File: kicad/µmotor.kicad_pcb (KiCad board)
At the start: 2 copper layers, 20 x 20 mm, 31 parts, among them J101 CAN+PWR, J201 TX, J202 RX, J203 SWDIO, J204 SWCLK, J205 GND, J501 1, J502 2, U201 STM32F042F6Px, U301 MCP1700T-3002E/TT, U401 AS5045B, U501 DRV8870, U502 INA180A1, U601 TCAN330

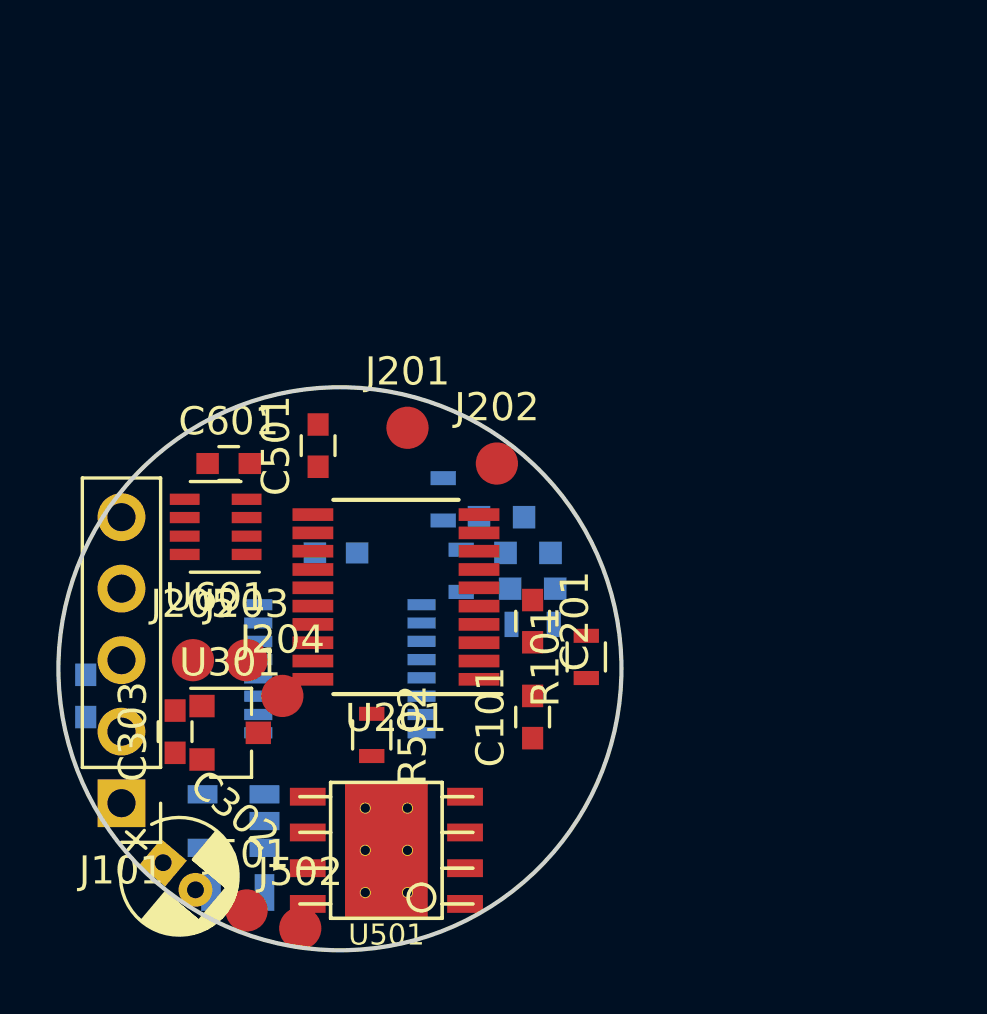
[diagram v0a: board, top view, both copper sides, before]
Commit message: layout: components placed
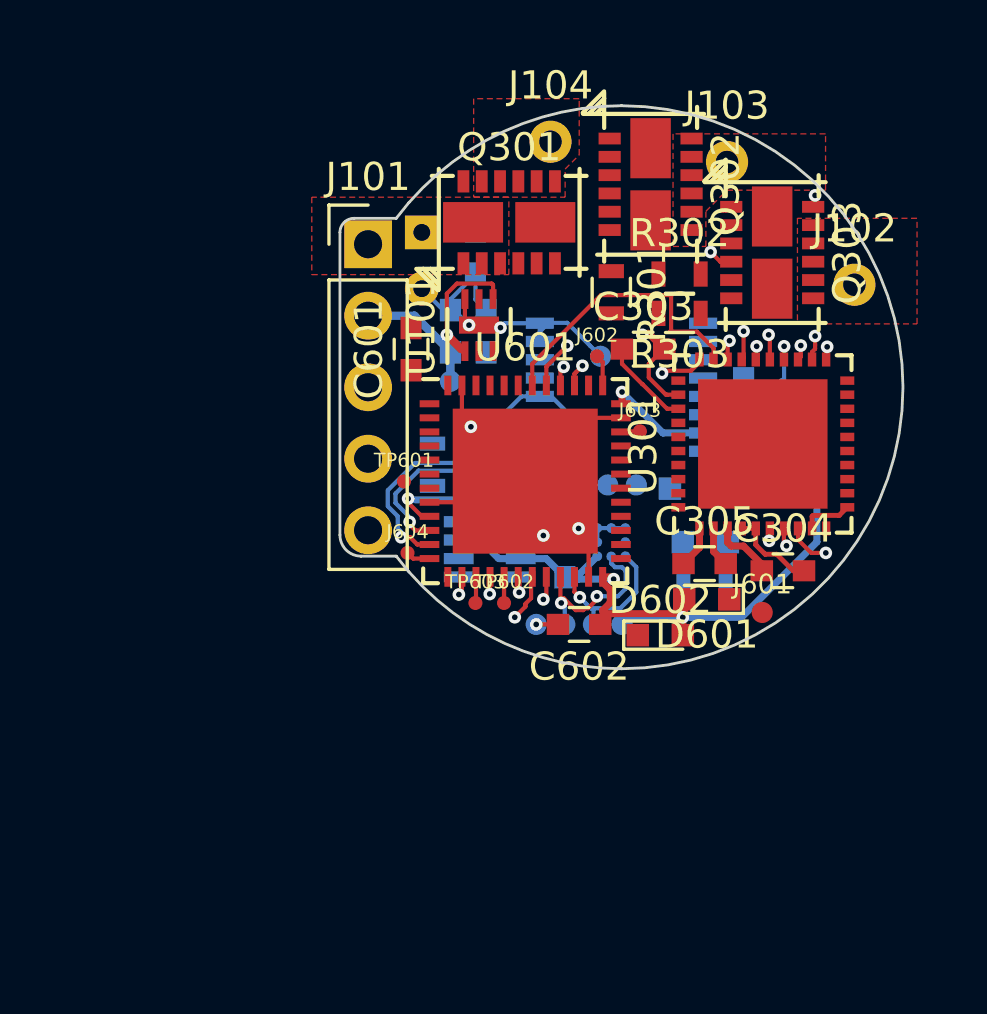
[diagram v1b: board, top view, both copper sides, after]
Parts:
- removed C501: NC, Capacitors_SMD:C_0603
- removed D401: Red, LEDs:LED_0603
- removed D402: Yellow, LEDs:LED_0603
- removed J205: GND, Measurement_Points:Measurement_Point_Round-SMD-Pad_Small
- removed R101: 100k, Resistors_SMD:R_0603
- removed R401, R402: 1k, Resistors_SMD:R_0603
- removed R501: 150m, Resistors_SMD:R_0805
- removed R502: 0, Resistors_SMD:R_0603
- removed U502: INA180A1, TO_SOT_Packages_SMD:SOT-23-5
- added C102: 1µ 6V3, Capacitors_SMD:C_0603, B.Cu at (155.2, 88.0)
- added C304: 1µ 16V X7R, Capacitors_SMD:C_0603, F.Cu at (165.7, 96.5)
- added C305: 47n 50V X7R, Capacitors_SMD:C_0603, F.Cu at (163.0, 96.3)
- added C602: 100n, Capacitors_SMD:C_0603, F.Cu at (158.5, 98.4)
- added D202: Yellow, LEDs:LED_0603, B.Cu at (162.5, 93.6)
- added D601: Blue, LEDs:LED_0603, F.Cu at (163.0, 97.5)
- added D602: Red, LEDs:LED_0603, F.Cu at (161.4, 98.8)
- added J102: U, Measurement_Points:Measurement_Point_Round-TH_Small, F.Cu at (168.3, 86.4)
- added J103: V, Measurement_Points:Measurement_Point_Round-TH_Small, F.Cu at (163.8, 82.0)
- added J104: W, Measurement_Points:Measurement_Point_Round-TH_Small, F.Cu at (157.5, 81.3)
- added J105: U, Measurement_Point_Round-SMD-Pad_Smaller:Measurement_Point_Round-SMD-Pad_Smaller_0.75mm, B.Cu at (160.5, 93.5)
- added J106: V, Measurement_Point_Round-SMD-Pad_Smaller:Measurement_Point_Round-SMD-Pad_Smaller_0.75mm, B.Cu at (159.5, 93.5)
- added J107: W, Measurement_Point_Round-SMD-Pad_Smaller:Measurement_Point_Round-SMD-Pad_Smaller_0.75mm, B.Cu at (158.5, 93.5)
- added J503: 3V3, Measurement_Point_Round-SMD-Pad_Smaller:Measurement_Point_Round-SMD-Pad_Smaller_0.75mm, B.Cu at (160.0, 98.4)
- added J504: GND, Measurement_Point_Round-SMD-Pad_Smaller:Measurement_Point_Round-SMD-Pad_Smaller_0.75mm, B.Cu at (157.0, 98.4)
- added J601: GND, Measurement_Point_Round-SMD-Pad_Smaller:Measurement_Point_Round-SMD-Pad_Smaller_0.75mm, F.Cu at (165.0, 98.0)
- added J602: SWCLK, Measurement_Point_Round-SMD-Pad_Smaller:Measurement_Point_Round-SMD-Pad_Smaller_0.5mm, F.Cu at (159.1, 88.9)
- added J603: SWDIO, Measurement_Point_Round-SMD-Pad_Smaller:Measurement_Point_Round-SMD-Pad_Smaller_0.5mm, F.Cu at (160.7, 91.6)
- added J604: TX, Measurement_Point_Round-SMD-Pad_Smaller:Measurement_Point_Round-SMD-Pad_Smaller_0.5mm, F.Cu at (152.4, 95.9)
- added Q301: FDMD82xx, DFN-12-2EP_3.3x5mm_Pitch0.65mm:DFN-12-2EP_3.3x5mm_Pitch0.65mm, F.Cu at (156.0, 84.1)
- added Q302: FDMD82xx, DFN-12-2EP_3.3x5mm_Pitch0.65mm:DFN-12-2EP_3.3x5mm_Pitch0.65mm, F.Cu at (161.0, 82.8)
- added Q303: FDMD82xx, DFN-12-2EP_3.3x5mm_Pitch0.65mm:DFN-12-2EP_3.3x5mm_Pitch0.65mm, F.Cu at (165.4, 85.2)
- added R202: 1k, Resistors_SMD:R_0603, B.Cu at (164.7, 93.1)
- added R301: 5m, Resistors_SMD:R_0603, F.Cu at (159.6, 86.6)
- added R302: 5m, Resistors_SMD:R_0603, F.Cu at (162.1, 86.0)
- added R303: 5m, Resistors_SMD:R_0603, F.Cu at (162.1, 87.4)
- added R601: 1k, Resistors_SMD:R_0603, B.Cu at (163.0, 96.9)
- added R602: 1k, Resistors_SMD:R_0603, B.Cu at (153.3, 92.8)
- added TP601: ~RST, Measurement_Point_Round-SMD-Pad_Smaller:Measurement_Point_Round-SMD-Pad_Smaller_0.5mm, F.Cu at (152.3, 93.3)
- added TP602: BK, Measurement_Point_Round-SMD-Pad_Smaller:Measurement_Point_Round-SMD-Pad_Smaller_0.5mm, F.Cu at (155.8, 97.7)
- added TP603: DAC, Measurement_Point_Round-SMD-Pad_Smaller:Measurement_Point_Round-SMD-Pad_Smaller_0.5mm, F.Cu at (154.8, 97.7)
- added U101: NCP4623HMX033TCG, Housings_DFN_QFN:DFN-6-1EP_2x2mm_Pitch0.5mm, F.Cu at (154.9, 87.8)
- C101: value 1u -> 1µ 16V; moved to B.Cu
- C201: moved to B.Cu
- C301: value 10µ/10V -> >10µ 35V; footprint Capacitors_SMD:C_0603 -> Capacitors_THT:CP_Radial_D4.0mm_P2.00mm
- C302: value 47µ/35V -> 100n 50V; footprint Capacitors_THT:CP_Radial_D4.0mm_P1.50mm -> Capacitors_SMD:C_0603; moved to B.Cu
- C303: value 10µ/6V3 -> 1µ 6V3 X7R
- D201: value Blue -> Red
- J201: value TX -> A; footprint Measurement_Points:Measurement_Point_Round-SMD-Pad_Small -> Measurement_Point_Round-SMD-Pad_Smaller:Measurement_Point_Round-SMD-Pad_Smaller_0.75mm; moved to B.Cu
- J202: value RX -> B; footprint Measurement_Points:Measurement_Point_Round-SMD-Pad_Small -> Measurement_Point_Round-SMD-Pad_Smaller:Measurement_Point_Round-SMD-Pad_Smaller_0.75mm; moved to B.Cu
- J203: value SWDIO -> 6V; footprint Measurement_Points:Measurement_Point_Round-SMD-Pad_Small -> Measurement_Point_Round-SMD-Pad_Smaller:Measurement_Point_Round-SMD-Pad_Smaller_0.75mm; moved to B.Cu
- J204: value SWCLK -> GND; footprint Measurement_Points:Measurement_Point_Round-SMD-Pad_Small -> Measurement_Point_Round-SMD-Pad_Smaller:Measurement_Point_Round-SMD-Pad_Smaller_0.75mm; moved to B.Cu
- J501: value 1 -> SCL; footprint Measurement_Points:Measurement_Point_Round-SMD-Pad_Small -> Measurement_Point_Round-SMD-Pad_Smaller:Measurement_Point_Round-SMD-Pad_Smaller_0.75mm; moved to B.Cu
- J502: value 2 -> SDA; footprint Measurement_Points:Measurement_Point_Round-SMD-Pad_Small -> Measurement_Point_Round-SMD-Pad_Smaller:Measurement_Point_Round-SMD-Pad_Smaller_0.75mm; moved to B.Cu
- U201: value STM32F042F6Px -> AS5045B; footprint Housings_SSOP:TSSOP-20_4.4x6.5mm_Pitch0.65mm -> Housings_SSOP:SSOP-16_4.4x5.2mm_Pitch0.65mm; moved to B.Cu
- U301: value MCP1700T-3002E/TT -> DRV8323S; footprint TO_SOT_Packages_SMD:SOT-23 -> Housings_DFN_QFN:QFN-40-1EP_6x6mm_Pitch0.5mm
- U401: value AS5045B -> TCAN330; footprint Housings_SSOP:SSOP-16_4.4x5.2mm_Pitch0.65mm -> TO_SOT_Packages_SMD:SOT-23-8
- U501: value DRV8870 -> TMP006; footprint HSOP-8:HSOP-8 -> WCSP-8_1.6x1.6mm_P0.5mm:WCSP-8_1.6x1.6mm_P0.5mm; moved to B.Cu
- U601: value TCAN330 -> STM32L433C(B-C)Ux_u; footprint TO_SOT_Packages_SMD:SOT-23-8 -> Housings_DFN_QFN:QFN-48-1EP_7x7mm_Pitch0.5mm
- moved C302 24.3 mm to (154.8, 85.2), turned to 270 degrees
- moved J101 21.7 mm to (151.0, 84.9), turned to 0 degrees
- moved U301 21.5 mm to (165.0, 92.0), turned to 90 degrees
- moved C303 21.5 mm to (160.8, 88.6), turned to 0 degrees
- moved C301 20.3 mm to (152.9, 84.5), turned to 270 degrees
- moved J204 16.5 mm to (159.3, 88.9)
- moved J501 15.2 mm to (158.0, 98.4)
- moved J502 15.0 mm to (159.0, 98.4)
- moved C101 14.0 mm to (153.9, 88.0)
- moved U501 13.6 mm to (159.6, 95.5), turned to 270 degrees
- moved J203 12.3 mm to (153.9, 89.8)
- moved U601 11.1 mm to (156.6, 93.3), turned to 0 degrees
- moved U201 10.9 mm to (160.0, 90.0), turned to 0 degrees
- moved C201 10.9 mm to (164.3, 90.4), turned to 90 degrees
- moved R201 10.8 mm to (166.2, 93.1), turned to 270 degrees
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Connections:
- C101 pad 1: /Motor_Driver/VREF -> +6V
- C301 pad 1: +6V -> +24V
- C303 pad 1: +3V3 -> /Motor_Driver/3V3_DRV
- D201 pad 2: +3V3 -> Net-(D201-Pad2)
- J201 pad 1: Net-(J201-Pad1) -> /Encoder/A
- J202 pad 1: Net-(J202-Pad1) -> /Encoder/B
- J203 pad 1: Net-(J203-Pad1) -> +6V
- J204 pad 1: Net-(J204-Pad1) -> GND
- J501 pad 1: Net-(J501-Pad1) -> /Microcontroller/I2C_SCL
- J502 pad 1: Net-(J502-Pad1) -> /Microcontroller/I2C_SDA
- R201 pad 1: Net-(R201-Pad1) -> +3V3
- R201 pad 2: Net-(D201-Pad1) -> Net-(D201-Pad2)
- U201 pad 1: (no net) -> Net-(D202-Pad1)
- U201 pad 10: /Microcontroller/PWM_TIM14_CH1 -> (no net)
- U201 pad 11: /Microcontroller/ADC -> (no net)
- U201 pad 13: /Motor_Driver/IN2 -> (no net)
- U201 pad 14: /Motor_Driver/IN1 -> (no net)
- U201 pad 15: GND -> +3V3
- U201 pad 2: (no net) -> Net-(D201-Pad1)
- U201 pad 3: Net-(R201-Pad1) -> /Encoder/A
- U201 pad 4: (no net) -> /Encoder/B
- U201 pad 5: +3V3 -> (no net)
- U201 pad 6: /Encoder/A -> (no net)
- U201 pad 7: /Encoder/B -> GND
- U201 pad 8: Net-(J201-Pad1) -> GND
- U201 pad 9: Net-(J202-Pad1) -> (no net)
- U301 pad 1: GND -> /Motor_Driver/CPL
- U301 pad 2: +3V3 -> /Motor_Driver/CPH
- U301 pad 3: +6V -> /Motor_Driver/VCP
- U401 pad 1: Net-(D402-Pad1) -> /CAN/CAN_TX
- U401 pad 2: Net-(D401-Pad1) -> GND
- U401 pad 3: /Encoder/A -> +3V3
- U401 pad 4: /Encoder/B -> /CAN/CAN_RX
- U401 pad 6: (no net) -> /CAN/CAN_L
- U401 pad 7: GND -> /CAN/CAN_H
- U401 pad 8: GND -> (no net)
- U601 pad 1: /CAN/CAN_TX -> +3V3
- U601 pad 2: GND -> (no net)
- U601 pad 3: +3V3 -> (no net)
- U601 pad 4: /CAN/CAN_RX -> (no net)
- U601 pad 5: (no net) -> /Microcontroller/LedRed
- U601 pad 6: /CAN/CAN_L -> (no net)
- U601 pad 7: /CAN/CAN_H -> /Microcontroller/~RST
- U601 pad 8: (no net) -> GND
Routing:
- net +3V3: track 0.00 -> 42.4 mm, vias 0 -> 5
- net GND: track 0.00 -> 28.2 mm, vias 0 -> 7
- net Net-(Q303-Pad4): track 0.00 -> 20.6 mm, vias 0 -> 2
- net /Microcontroller/GpioB2: track 0.00 -> 19.3 mm, vias 0 -> 2
- net /Motor_Driver/ENABLE: track 0.00 -> 17.3 mm, vias 0 -> 2
- net /Microcontroller/SenseV: track 0.00 -> 17.1 mm, vias 0 -> 2
- net /Microcontroller/SenseAll: track 0.00 -> 17.0 mm, vias 0 -> 2
- net /Microcontroller/SenseW: track 0.00 -> 15.8 mm, vias 0 -> 2
- net Net-(Q303-Pad12): track 0.00 -> 15.4 mm, vias 0 -> 2
- net /Motor_Driver/OUT_U: track 0.00 -> 11.8 mm, vias 0 -> 1
- net /Encoder/B: track 0.00 -> 11.6 mm, vias 0 -> 1
- net /Encoder/A: track 0.00 -> 10.7 mm, vias 0 -> 1
- net /Microcontroller/CS: track 0.00 -> 10.2 mm
- net +6V: track 0.00 -> 9.84 mm, vias 0 -> 1
- net /Microcontroller/MOSI: track 0.00 -> 9.70 mm, vias 0 -> 2
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- added copper zone on F.Cu, net +24V
- added copper zone on In1.Cu, net +24V
- added copper zone on F.Cu, net /Motor_Driver/OUT_U
- added copper zone on F.Cu, net /Motor_Driver/OUT_V
- added copper zone on F.Cu, net /Motor_Driver/OUT_W
- added copper zone on In1.Cu, net GND
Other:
- outline, holes or cut-outs redrawn
- copper layers 2 -> 4
- net class Default: clearance 0.2 -> 0.125; trace_width 0.25 -> 0.15; via_dia 0.6 -> 0.45; via_drill 0.4 -> 0.2
- rule pad_to_mask_clearance: 0.05 -> 0
- rule trace_clearance: 0.2 -> 0.125
- rule trace_min: 0.2 -> 0.1
- rule via_min_drill: 0.3 -> 0.2
- rule via_min_size: 0.4 -> 0.45

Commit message: layout: routing finished
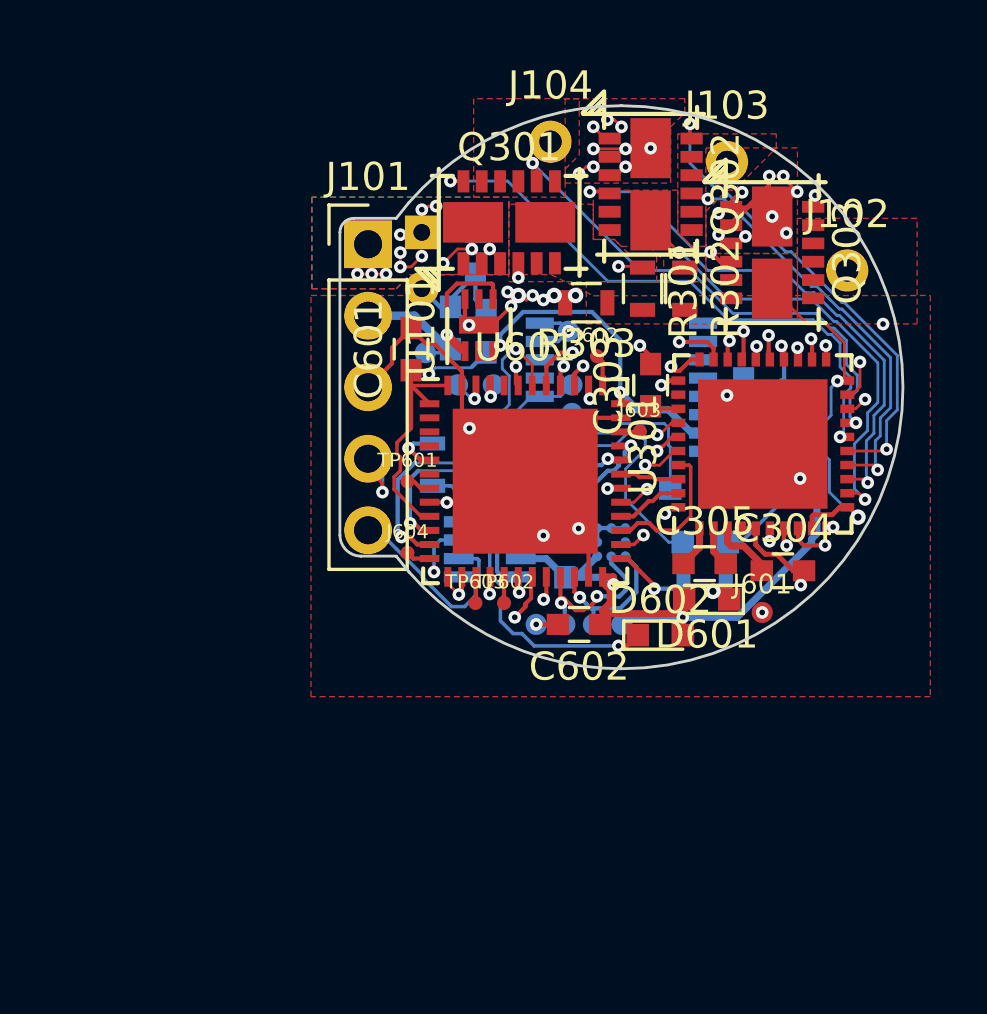
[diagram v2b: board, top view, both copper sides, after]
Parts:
- moved J105 7.28 mm to (154.2, 89.9)
- moved J106 5.40 mm to (155.4, 89.9)
- moved J107 3.72 mm to (155.4, 91.4)
- moved R303 3.34 mm to (158.8, 87.0)
- moved D202 1.96 mm to (163.0, 95.5)
- moved D201 1.96 mm to (162.5, 93.6)
- moved R201 1.52 mm to (164.7, 93.1)
- moved J204 1.45 mm to (158.1, 88.0)
- moved J202 1.42 mm to (158.2, 89.9)
- moved J201 1.42 mm to (158.2, 90.9)
- moved R202 1.40 mm to (166.1, 93.1)
- moved J203 1.35 mm to (153.0, 88.8)
- moved C303 1.31 mm to (161.0, 89.9), turned to 90 degrees
- moved R301 1.12 mm to (160.8, 86.5)
- moved J102 0.57 mm to (168.0, 85.9)
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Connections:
- U601 pad 32: /Microcontroller/HallV -> /CAN/CAN_RX
- U601 pad 33: /Microcontroller/HallU -> /CAN/CAN_TX
- U601 pad 38: /Microcontroller/HallW -> /Microcontroller/CS
- U601 pad 42: /Microcontroller/CS -> /Microcontroller/HallW
- U601 pad 45: /CAN/CAN_RX -> /Microcontroller/HallV
- U601 pad 46: /CAN/CAN_TX -> /Microcontroller/HallU
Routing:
- net +24V: track 3.18 -> 53.9 mm, vias 0 -> 32
- net GND: track 28.2 -> 67.0 mm, vias 7 -> 20
- net Net-(Q301-Pad12): track 0.00 -> 20.6 mm, vias 0 -> 2
- net Net-(Q302-Pad4): track 0.00 -> 19.2 mm, vias 0 -> 2
- net /Motor_Driver/OUT_W: track 0.00 -> 18.0 mm, vias 0 -> 2
- net Net-(Q302-Pad12): track 0.00 -> 17.0 mm, vias 0 -> 2
- net Net-(Q301-Pad4): track 0.00 -> 16.4 mm, vias 0 -> 2
- net Net-(Q302-Pad14): track 0.00 -> 16.3 mm, vias 0 -> 2
- net /Motor_Driver/OUT_V: track 0.00 -> 14.2 mm, vias 0 -> 2
- net +3V3: track 42.4 -> 56.3 mm, vias 5 -> 6
- net Net-(Q301-Pad14): track 0.00 -> 12.7 mm, vias 0 -> 2
- net /Microcontroller/LedRedR: track 0.00 -> 11.7 mm, vias 0 -> 1
- net Net-(Q303-Pad14): track 1.81 -> 13.0 mm, vias 0 -> 2
- net /Microcontroller/GpioB7: track 0.00 -> 10.8 mm, vias 0 -> 2
- net Net-(D202-Pad1): track 0.00 -> 9.21 mm
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- added copper zone on B.Cu, net +24V
- added copper zone on F.Cu, net GND
- added copper zone on F.Cu, net Net-(Q301-Pad14)
- added copper zone on F.Cu, net Net-(Q302-Pad14)
- added copper zone on F.Cu, net Net-(Q303-Pad14)
